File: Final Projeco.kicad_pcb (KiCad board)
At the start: 2 copper layers, 25 x 45 mm, 16 parts, among them U1 ESP32-S3, U2 GT-USB-7004N, U3 NCP167BMX330TBG, X1 TZ1269D

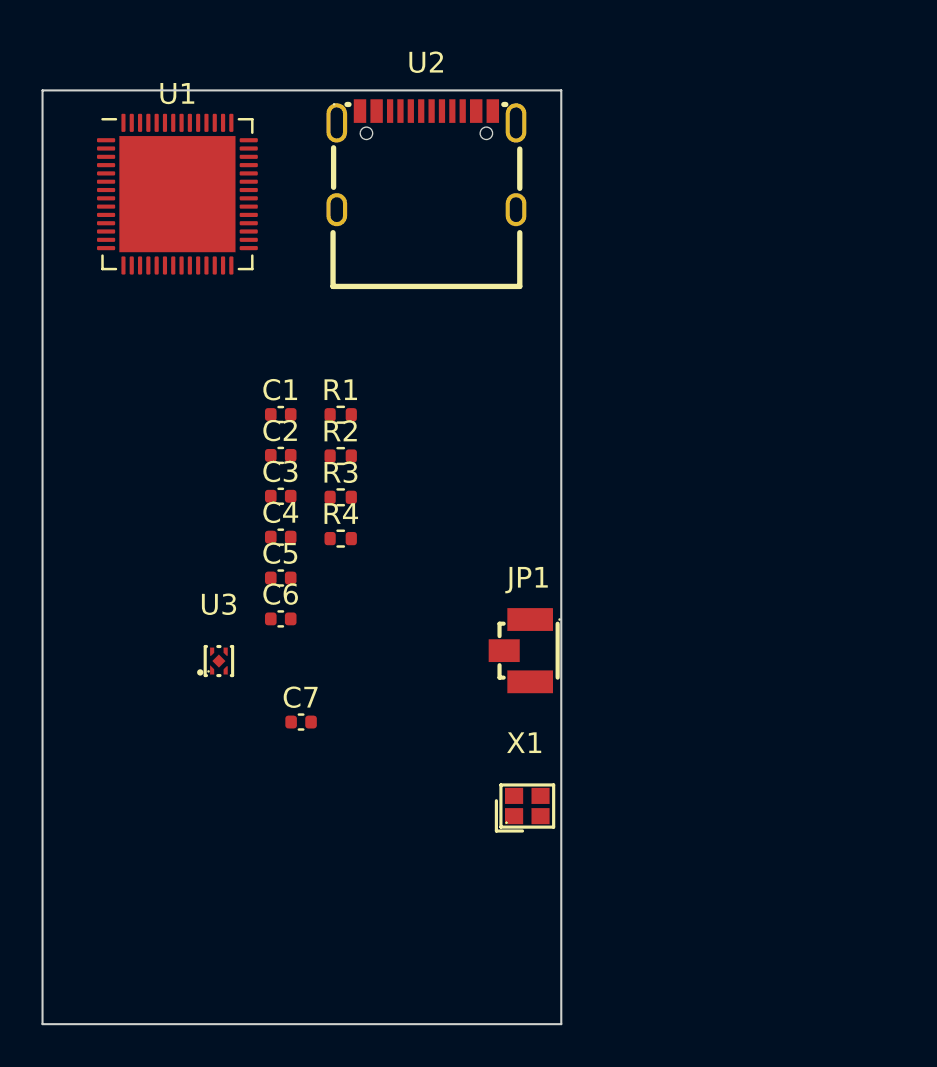
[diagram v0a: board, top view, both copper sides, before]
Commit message: Fixed all the traces to connect to each other :-|
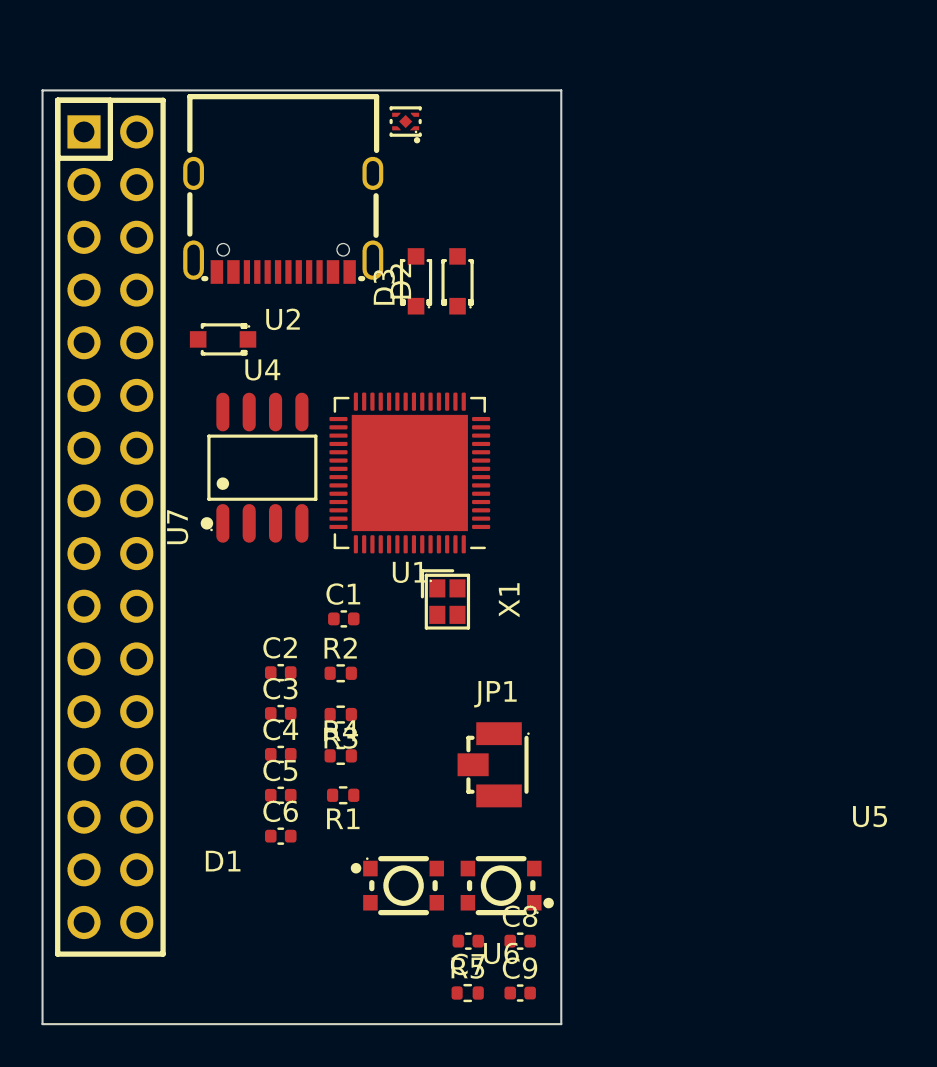
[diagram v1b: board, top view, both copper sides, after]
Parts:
- added C8: 1uF, Capacitor_SMD:C_0402_1005Metric, F.Cu at (49.5, 56.5)
- added C9: 0.1uF, Capacitor_SMD:C_0402_1005Metric, F.Cu at (49.5, 59.0)
- added D1: SD103AWS_C5345966, jlc:SOD-323_L1.7-W1.3-LS2.5-RD, F.Cu at (35.2, 27.5)
- added D2: SD103AWS_C5345966, jlc:SOD-323_L1.7-W1.3-LS2.5-RD, F.Cu at (46.5, 24.7)
- added D3: SD103AWS_C5345966, jlc:SOD-323_L1.7-W1.3-LS2.5-RD, F.Cu at (44.5, 24.7)
- added R5: 100K, Resistor_SMD:R_0402_1005Metric, F.Cu at (47.0, 59.0)
- added U4: LY68L6400SLIT, jlc:SOP-8_L4.9-W3.9-P1.27-LS6.0-BL, F.Cu at (37.1, 33.7)
- added U5: PTS830GG140SMTRLFS, jlc:KEY-SMD_4P-L3.1-W2.6_PTS830GG140SMTRLFS, F.Cu at (43.9, 53.8)
- added U6: PTS830GG140SMTRLFS, jlc:KEY-SMD_4P-L3.1-W2.6_PTS830GG140SMTRLFS, F.Cu at (48.6, 53.8)
- added U7: 220S-2*16P_H=8_5MM_Ytype_L=3_0MM_PBT, jlc:HDR-TH_32P-P2.54-V-F-R2-C16-S2.54, F.Cu at (29.8, 36.6)
- C4: value C -> 1u
- moved U3 27.5 mm to (44.0, 17.0), turned to 90 degrees
- moved R1 18.3 mm to (41.0, 49.5), turned to 180 degrees
- moved U1 17.5 mm to (44.2, 33.9), turned to 180 degrees
- moved C7 13.3 mm to (47.0, 56.5), turned to 180 degrees
- moved X1 10.6 mm to (46.0, 40.1), turned to -90 degrees
- moved R2 10.5 mm to (40.9, 43.6)
- moved C2 10.5 mm to (38.0, 43.6)
- moved C3 10.5 mm to (38.0, 45.5)
- moved C4 10.5 mm to (38.0, 47.5)
- moved C5 10.5 mm to (38.0, 49.5)
- moved C6 10.5 mm to (38.0, 51.4)
- moved R3 10.5 mm to (40.9, 45.6), turned to 180 degrees
- moved R4 10.5 mm to (40.9, 47.6)
- moved C1 10.3 mm to (41.0, 41.0)
- moved U2 7.53 mm to (38.1, 21.9), turned to 180 degrees
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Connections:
- C1 pad 2: Net-(C1-Pad2) -> /XTAL_P
- C2 pad 1: Net-(C2-Pad1) -> /XTAL_N
- C3 pad 1: Net-(C3-Pad1) -> /RESET
- C5 pad 1: Net-(U3-OUT) -> VDD3P3
- C6 pad 1: Net-(U3-EN) -> /VBUS
- R1 pad 2: Net-(C3-Pad1) -> /RESET
- R2 pad 1: Net-(U2-CC2) -> /VBUS
- R3 pad 1: Net-(U2-CC1) -> /VBUS
- U1 pad 10: unconnected-(U1-GPIO5/ADC1_CH4-Pad10) -> /GPIO5
- U1 pad 11: unconnected-(U1-GPIO6/ADC1_CH5-Pad11) -> /GPIO6
- U1 pad 12: unconnected-(U1-GPIO7/ADC1_CH6-Pad12) -> /GPIO7
- U1 pad 13: unconnected-(U1-GPIO8/ADC1_CH7-Pad13) -> /GPIO8
- U1 pad 14: unconnected-(U1-GPIO9/ADC1_CH8-Pad14) -> /GPIO9'
- U1 pad 15: unconnected-(U1-GPIO10/ADC1_CH9-Pad15) -> /GPIO10
- U1 pad 16: unconnected-(U1-GPIO11/ADC2_CH0-Pad16) -> /GPIO11
- U1 pad 17: unconnected-(U1-GPIO12/ADC2_CH1-Pad17) -> /GPIO12
- U1 pad 18: unconnected-(U1-GPIO13/ADC2_CH2-Pad18) -> /GPIO13
- U1 pad 19: unconnected-(U1-GPIO14/ADC2_CH3-Pad19) -> /GPIO14
- U1 pad 20: unconnected-(U1-VDD3P3_RTC-Pad20) -> VDD3P3
- U1 pad 23: unconnected-(U1-GPIO17/ADC2_CH6-Pad23) -> /GPIO!7
- U1 pad 24: unconnected-(U1-GPIO18/ADC2_CH7-Pad24) -> /GPIO18
- U1 pad 25: unconnected-(U1-GPIO19/USB_D-/ADC2_CH8-Pad25) -> /USB_D+
- U1 pad 26: unconnected-(U1-GPIO20/USB_D+/ADC2_CH9-Pad26) -> /USB_D-
- U1 pad 27: unconnected-(U1-GPIO21-Pad27) -> /GPIO21
- U1 pad 28: unconnected-(U1-SPI_CS1/GPIO26-Pad28) -> /SPICS1
- U1 pad 29: unconnected-(U1-VDD_SPI-Pad29) -> VDD3P3
- U1 pad 30: unconnected-(U1-SPIHD/GPIO27-Pad30) -> /SPIHD
- U1 pad 31: unconnected-(U1-SPIWP/GPIO28-Pad31) -> /SPIWP
- U1 pad 33: unconnected-(U1-SPICLK/GPIO30-Pad33) -> /SPICLK
- U1 pad 34: unconnected-(U1-SPIQ/GPIO31-Pad34) -> /SPIQ
- U1 pad 35: unconnected-(U1-SPID/GPIO32-Pad35) -> /SPID
- U1 pad 4: unconnected-(U1-CHIP_PU/RESET-Pad4) -> /RESET
- U1 pad 43: unconnected-(U1-GPIO38-Pad43) -> /GPIO38
- U1 pad 46: unconnected-(U1-VDD3P3_CPU-Pad46) -> VDD3P3
- U1 pad 5: unconnected-(U1-GPIO0/BOOT-Pad5) -> /GPIO0/BOOT
- U1 pad 51: unconnected-(U1-GPIO45-Pad51) -> /GPIO45
- U1 pad 52: unconnected-(U1-GPIO46-Pad52) -> /GPIO46
- U1 pad 53: unconnected-(U1-XTAL_N-Pad53) -> /XTAL_P
- U1 pad 54: unconnected-(U1-XTAL_P-Pad54) -> /XTAL_N
- U1 pad 55: Net-(U1-VDDA-Pad55) -> VDD3P3
- U1 pad 56: Net-(U1-VDDA-Pad55) -> VDD3P3
- U1 pad 6: unconnected-(U1-GPIO1/ADC1_CH0-Pad6) -> /GPIO1
- U1 pad 7: unconnected-(U1-GPIO2/ADC1_CH1-Pad7) -> /GPIO2
- U1 pad 8: unconnected-(U1-GPIO3/ADC1_CH2-Pad8) -> /GPIO3
- U1 pad 9: unconnected-(U1-GPIO4/ADC1_CH3-Pad9) -> /GPIO4
- U2 pad 1: unconnected-(U2-SHELL-Pad1) -> GND
- U2 pad A4B9: Net-(U2-CC1) -> /VBUS
- U2 pad A5: Net-(U2-CC1) -> /VBUS
- U2 pad A6: unconnected-(U2-DP1-PadA6) -> /USB_D+
- U2 pad A7: unconnected-(U2-DN1-PadA7) -> /USB_D-
- U2 pad B4A9: Net-(U2-CC2) -> /VBUS
- U2 pad B5: Net-(U2-CC2) -> /VBUS
- U2 pad B6: unconnected-(U2-DP2-PadB6) -> /USB_D+
- U2 pad B7: unconnected-(U2-DN2-PadB7) -> /USB_D-
- U3 pad 1: Net-(U3-OUT) -> VDD3P3
- U3 pad 3: Net-(U3-EN) -> /VBUS
- U3 pad 4: Net-(U3-EN) -> /VBUS
- X1 pad 1: Net-(C1-Pad2) -> /XTAL_P
- X1 pad 3: Net-(C2-Pad1) -> /XTAL_N
